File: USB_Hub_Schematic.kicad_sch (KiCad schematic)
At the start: 125 parts, among them J1 USB-C, J2 USB-A, U1 USB2517 Chip, U10 TP, U11 TP, U12 TP, U13 TP, U14 TP, U15 TP, U16 TPS25821, U17 TPS25821, U2 USB to microSD, U3 MUX, U5 3.3V CONV, U7 TPS2052B, U9 TP, X1 24MHz, X2 24MHz

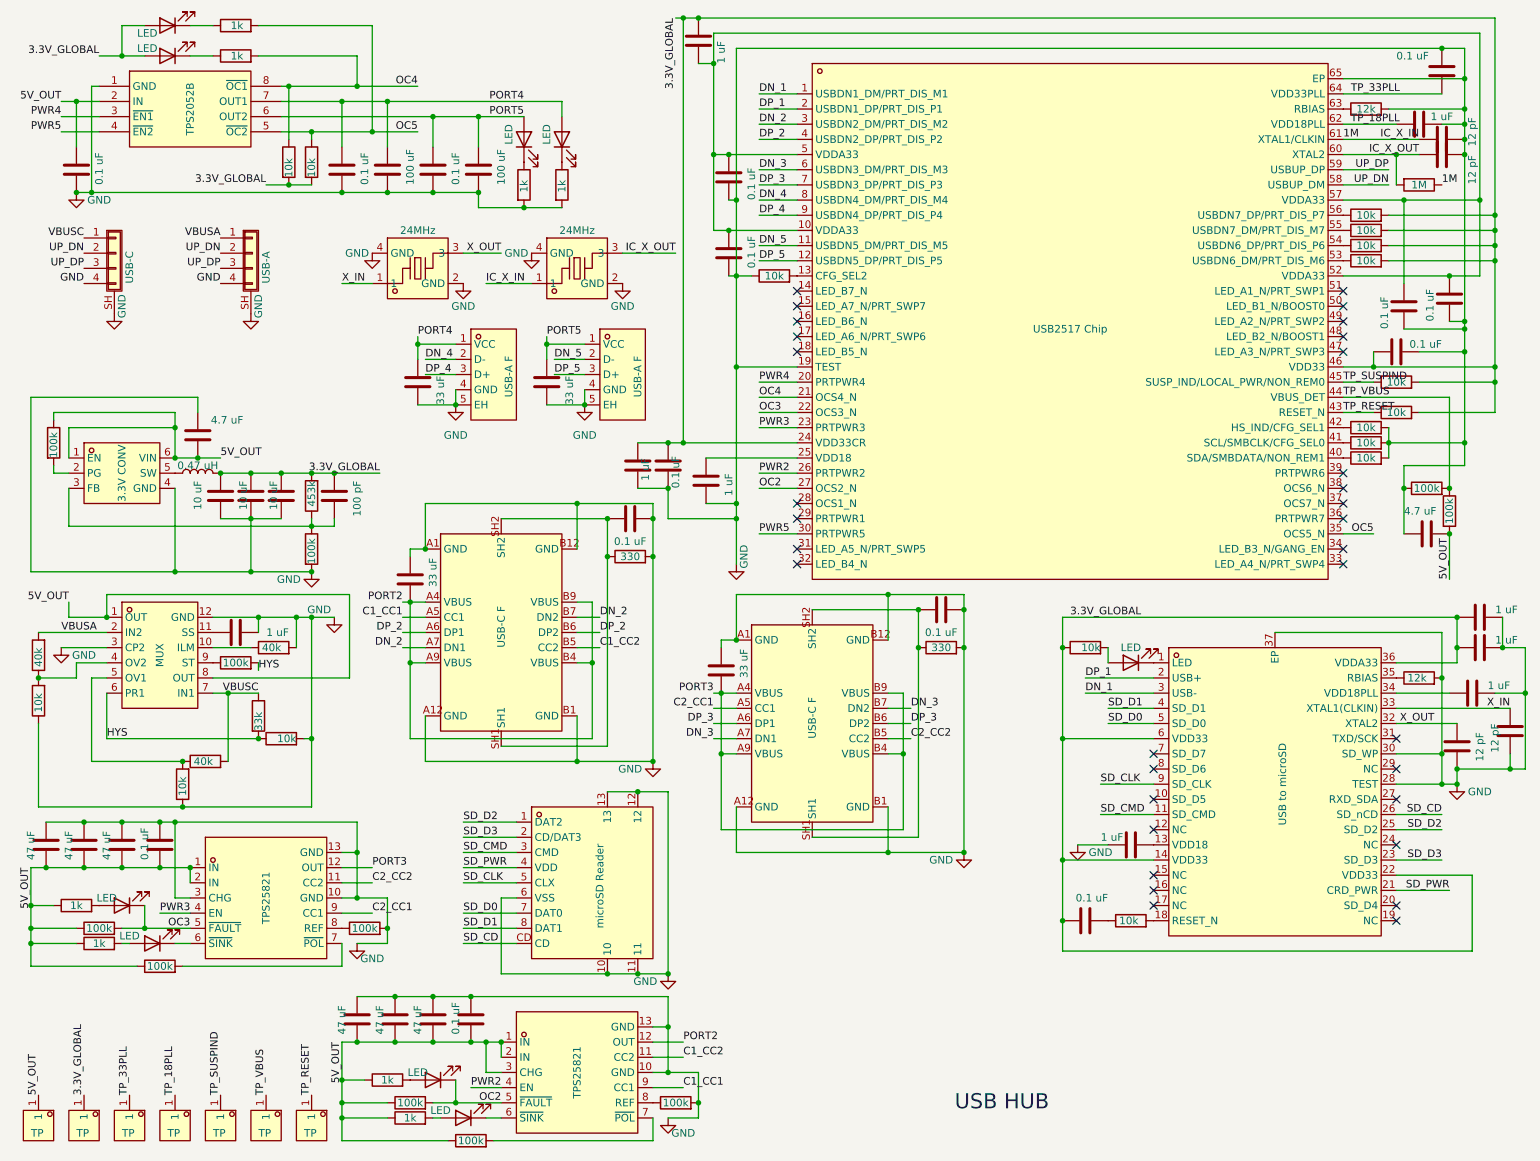
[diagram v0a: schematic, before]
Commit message: Routing
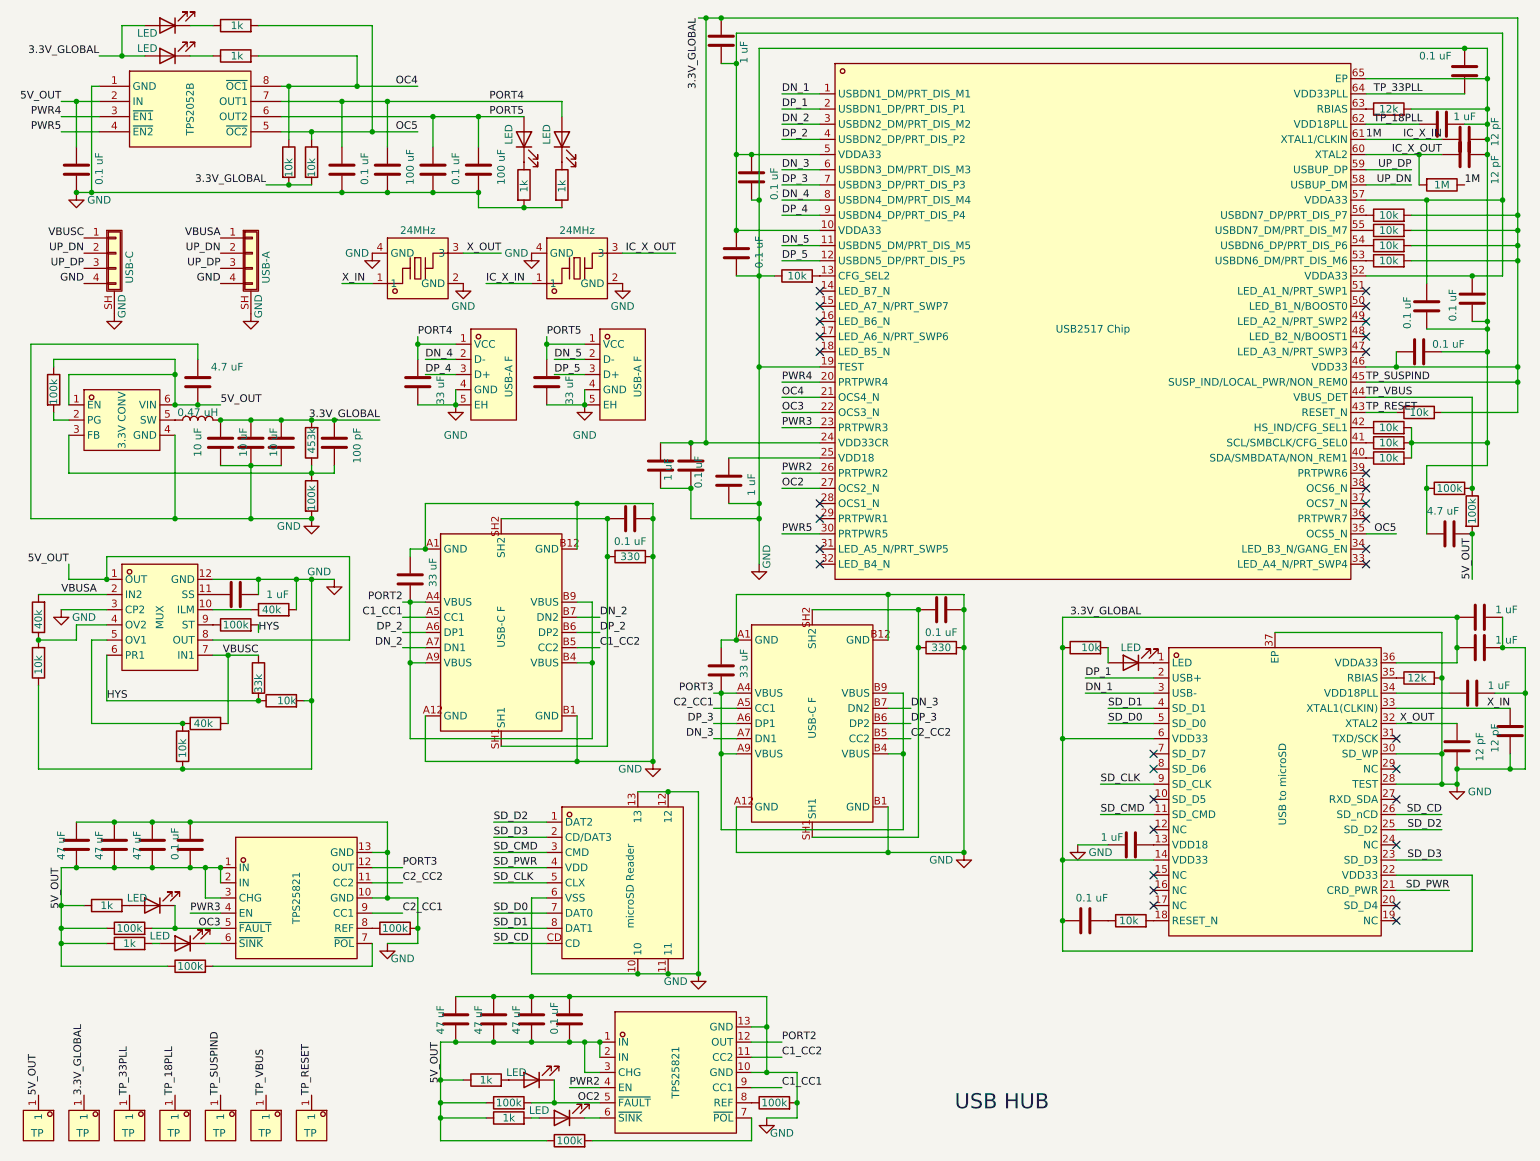
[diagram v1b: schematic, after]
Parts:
- removed R37: 10k, Resistor_SMD:R_0603_1608Metric, symbol Device:R
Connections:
- net TP_SUSPIND is gone; now on net 3.3V_GLOBAL: U1.45 (SUSP_IND/LOCAL_PWR/NON_REM0), U13.1
- net 5V_OUT: now also U17.3 (CHG)
- net GND: no longer U17.3 (CHG)
